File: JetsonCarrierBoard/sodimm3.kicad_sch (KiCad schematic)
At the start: 1 part

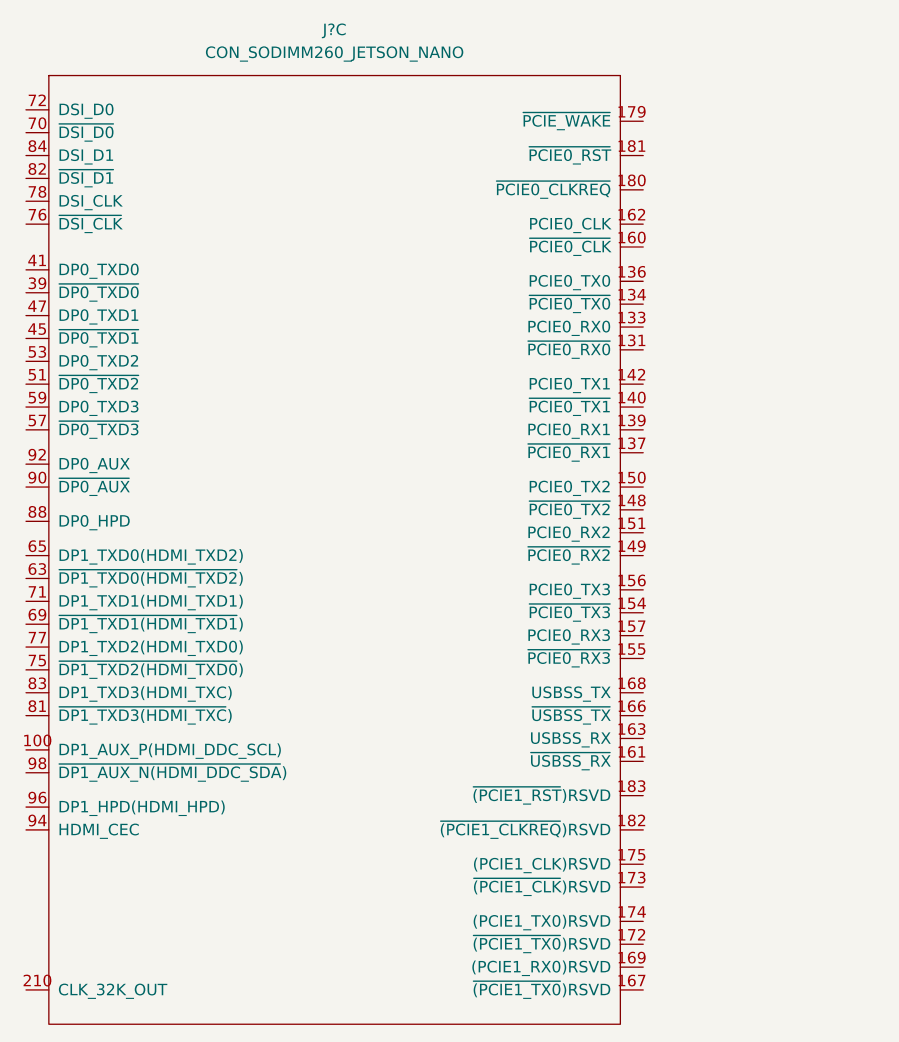
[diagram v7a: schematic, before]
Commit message: Finished Basic Wiring WiFi/BT V1
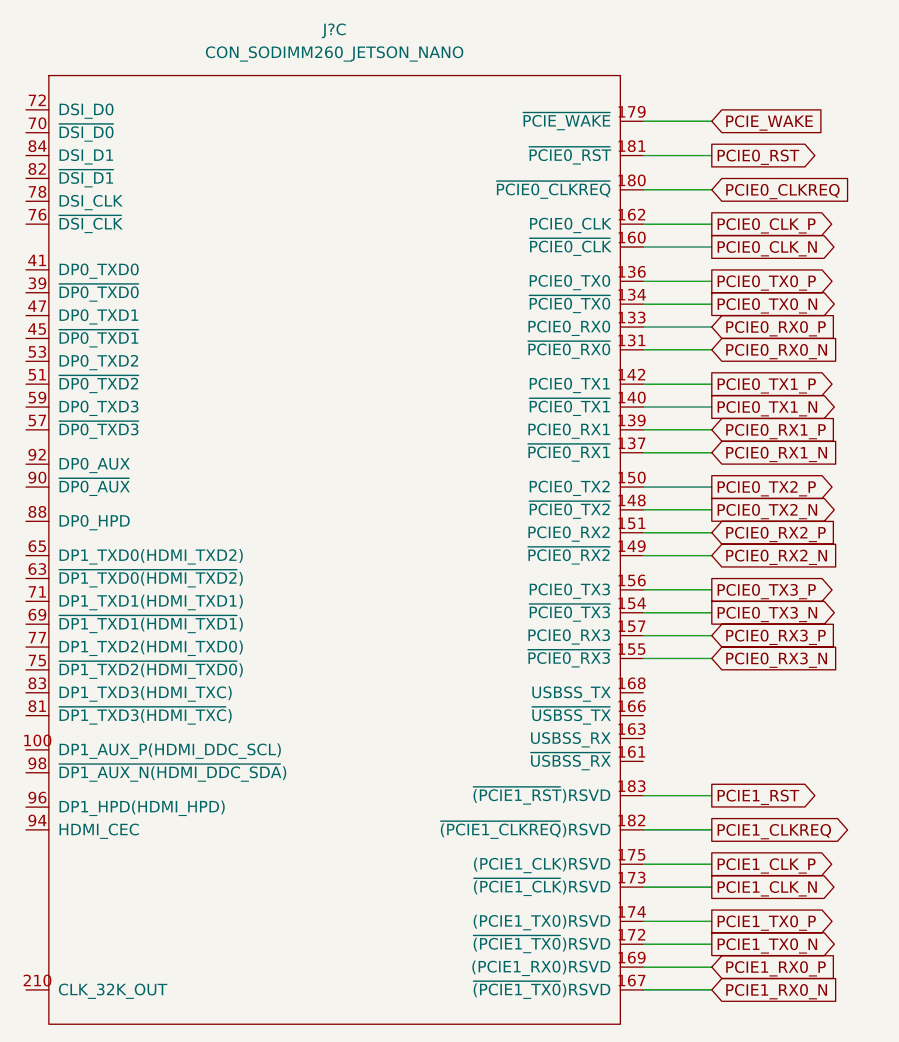
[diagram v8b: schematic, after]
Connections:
- net PCIE0_RX0_N: now reaches J?.131 (~{PCIE0_RX0})
- net PCIE0_RX0_P: now reaches J?.133 (PCIE0_RX0)
- net PCIE0_TX0_N: now reaches J?.134 (~{PCIE0_TX0})
- net PCIE0_TX0_P: now reaches J?.136 (PCIE0_TX0)
- net PCIE0_RX1_N: now reaches J?.137 (~{PCIE0_RX1})
- net PCIE0_RX1_P: now reaches J?.139 (PCIE0_RX1)
- net PCIE0_TX1_N: now reaches J?.140 (~{PCIE0_TX1})
- net PCIE0_TX1_P: now reaches J?.142 (PCIE0_TX1)
- net PCIE0_TX2_N: now reaches J?.148 (~{PCIE0_TX2})
- net PCIE0_RX2_N: now reaches J?.149 (~{PCIE0_RX2})
- net PCIE0_TX2_P: now reaches J?.150 (PCIE0_TX2)
- net PCIE0_RX2_P: now reaches J?.151 (PCIE0_RX2)
- net PCIE0_TX3_N: now reaches J?.154 (~{PCIE0_TX3})
- net PCIE0_RX3_N: now reaches J?.155 (~{PCIE0_RX3})
- net PCIE0_TX3_P: now reaches J?.156 (PCIE0_TX3)
- net PCIE0_RX3_P: now reaches J?.157 (PCIE0_RX3)
- net PCIE0_CLK_N: now reaches J?.160 (~{PCIE0_CLK})
- net PCIE0_CLK_P: now reaches J?.162 (PCIE0_CLK)
- net PCIE1_RX0_N: now reaches J?.167 (~{(PCIE1_TX0})RSVD)
- net PCIE1_RX0_P: now reaches J?.169 ((PCIE1_RX0)RSVD)
- net PCIE1_TX0_N: now reaches J?.172 (~{(PCIE1_TX0})RSVD)
- net PCIE1_CLK_N: now reaches J?.173 (~{(PCIE1_CLK})RSVD)
- net PCIE1_TX0_P: now reaches J?.174 ((PCIE1_TX0)RSVD)
- net PCIE1_CLK_P: now reaches J?.175 ((PCIE1_CLK)RSVD)
- net PCIE_WAKE: now reaches J?.179 (~{PCIE_WAKE})
- net PCIE0_CLKREQ: now reaches J?.180 (~{PCIE0_CLKREQ})
- net PCIE0_RST: now reaches J?.181 (~{PCIE0_RST})
- net PCIE1_CLKREQ: now reaches J?.182 (~{(PCIE1_CLKREQ})RSVD)
- net PCIE1_RST: now reaches J?.183 (~{(PCIE1_RST})RSVD)
